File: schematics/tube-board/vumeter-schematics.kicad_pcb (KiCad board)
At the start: 2 copper layers, 100 x 30 mm, 51 parts, among them J1 SWD, J2 Conn_01x04, J3 Conn_01x04, J4 Standoff_1, J5 Standoff_2, J6 Conn_01x01_Male, J7 Conn_01x01_Male, Q1 MJE340, Q2 MJE340, Q3 MJE340, Q4 MJE340, U1 LM358, U2 ATSAMD11C14, U3 LM1117-3.3, U4 LM358, U5 NCH8200HV, U6 NCH8200HV, U7 TPS2281DBVR

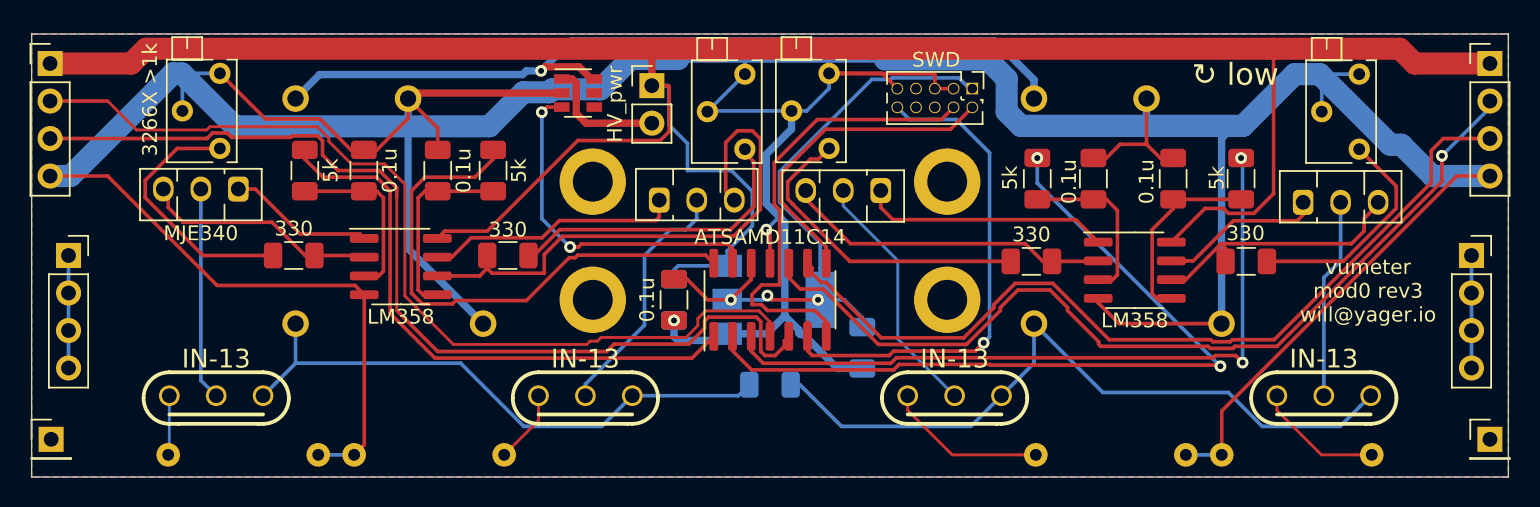
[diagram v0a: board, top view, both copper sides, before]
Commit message: ok
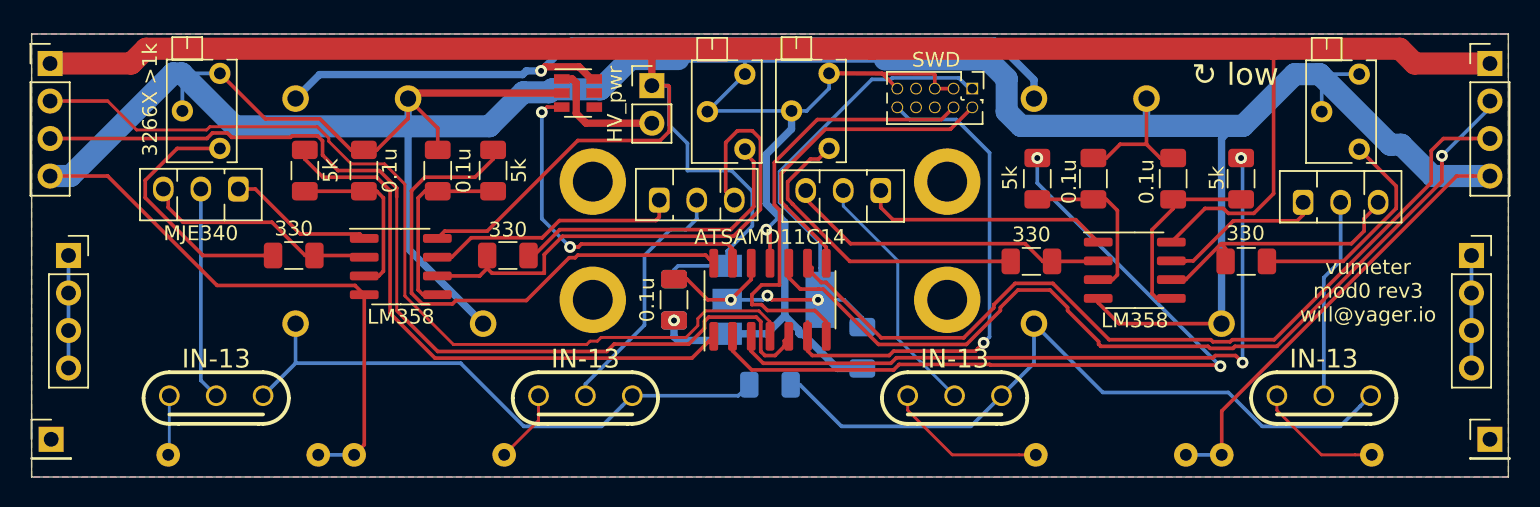
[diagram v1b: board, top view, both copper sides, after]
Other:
- net class 75V removed
- net class Default removed
- net class HV removed
